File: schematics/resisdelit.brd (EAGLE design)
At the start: 10 x 14 mm, 7 parts

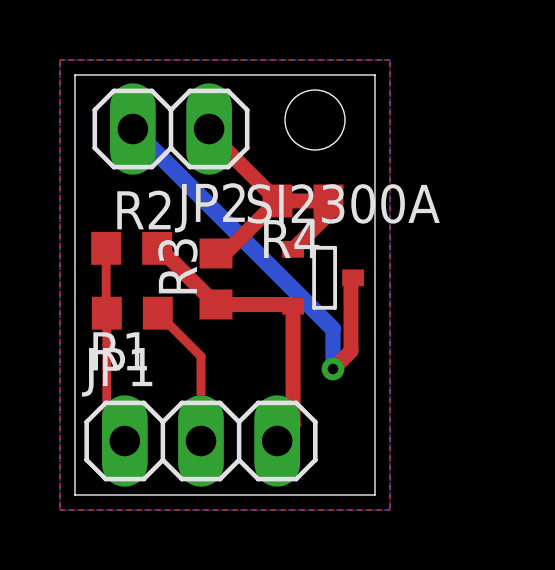
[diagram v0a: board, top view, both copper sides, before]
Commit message: заказ плат
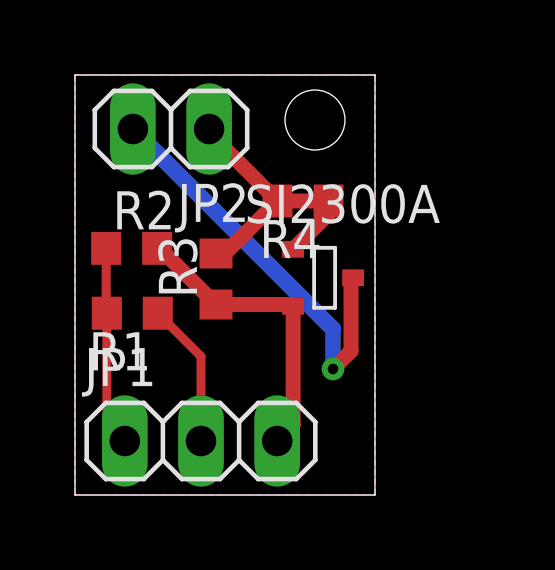
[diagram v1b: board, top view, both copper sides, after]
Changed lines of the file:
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@@
 <?xml version="1.0" encoding="utf-8"?>
 <!DOCTYPE eagle SYSTEM "eagle.dtd">
-<eagle version="9.6.2">
+<eagle version="9.4.2">
 <drawing>
 <settings>
-<setting alwaysvectorfont="no"/>
+<setting alwaysvectorfont="yes"/>
 <setting verticaltext="up"/>
 </settings>
@@
 <layer number="23" name="tOrigins" color="15" fill="1" visible="yes" active="yes"/>
 <layer number="24" name="bOrigins" color="15" fill="1" visible="yes" active="yes"/>
-<layer number="25" name="tNames" color="7" fill="1" visible="no" active="yes"/>
+<layer number="25" name="tNames" color="7" fill="1" visible="yes" active="yes"/>
 <layer number="26" name="bNames" color="7" fill="1" visible="yes" active="yes"/>
 <layer number="27" name="tValues" color="7" fill="1" visible="yes" active="yes"/>
 <layer number="28" name="bValues" color="7" fill="1" visible="yes" active="yes"/>
-<layer number="29" name="tStop" color="7" fill="3" visible="no" active="yes"/>
-<layer number="30" name="bStop" color="7" fill="6" visible="no" active="yes"/>
-<layer number="31" name="tCream" color="7" fill="4" visible="no" active="yes"/>
-<layer number="32" name="bCream" color="7" fill="5" visible="no" active="yes"/>
-<layer number="33" name="tFinish" color="6" fill="3" visible="no" active="yes"/>
-<layer number="34" name="bFinish" color="6" fill="6" visible="no" active="yes"/>
-<layer number="35" name="tGlue" color="7" fill="4" visible="no" active="yes"/>
-<layer number="36" name="bGlue" color="7" fill="5" visible="no" active="yes"/>
-<layer number="37" name="tTest" color="7" fill="1" visible="no" active="yes"/>
-<layer number="38" name="bTest" color="7" fill="1" visible="no" active="yes"/>
+<layer number="29" name="tStop" color="7" fill="3" visible="yes" active="yes"/>
+<layer number="30" name="bStop" color="7" fill="6" visible="yes" active="yes"/>
+<layer number="31" name="tCream" color="7" fill="4" visible="yes" active="yes"/>
+<layer number="32" name="bCream" color="7" fill="5" visible="yes" active="yes"/>
+<layer number="33" name="tFinish" color="6" fill="3" visible="yes" active="yes"/>
+<layer number="34" name="bFinish" color="6" fill="6" visible="yes" active="yes"/>
+<layer number="35" name="tGlue" color="7" fill="4" visible="yes" active="yes"/>
+<layer number="36" name="bGlue" color="7" fill="5" visible="yes" active="yes"/>
+<layer number="37" name="tTest" color="7" fill="1" visible="yes" active="yes"/>
+<layer number="38" name="bTest" color="7" fill="1" visible="yes" active="yes"/>
 <layer number="39" name="tKeepout" color="4" fill="11" visible="yes" active="yes"/>
 <layer number="40" name="bKeepout" color="1" fill="11" visible="yes" active="yes"/>
@@
 <layer number="42" name="bRestrict" color="1" fill="10" visible="yes" active="yes"/>
 <layer number="43" name="vRestrict" color="2" fill="10" visible="yes" active="yes"/>
-<layer number="44" name="Drills" color="7" fill="1" visible="no" active="yes"/>
+<layer number="44" name="Drills" color="7" fill="1" visible="yes" active="yes"/>
 <layer number="45" name="Holes" color="7" fill="1" visible="yes" active="yes"/>
-<layer number="46" name="Milling" color="3" fill="1" visible="no" active="yes"/>
-<layer number="47" name="Measures" color="7" fill="1" visible="no" active="yes"/>
+<layer number="46" name="Milling" color="3" fill="1" visible="yes" active="yes"/>
+<layer number="47" name="Measures" color="7" fill="1" visible="yes" active="yes"/>
 <layer number="48" name="Document" color="7" fill="1" visible="yes" active="yes"/>
 <layer number="49" name="Reference" color="7" fill="1" visible="yes" active="yes"/>
@@
 <layer number="111" name="111" color="7" fill="1" visible="no" active="no"/>
 <layer number="112" name="tSilk" color="7" fill="1" visible="no" active="no"/>
-<layer number="113" name="IDFDebug" color="7" fill="1" visible="no" active="yes"/>
+<layer number="113" name="IDFDebug" color="7" fill="1" visible="yes" active="yes"/>
 <layer number="114" name="Badge_Outline" color="7" fill="1" visible="no" active="no"/>
 <layer number="115" name="ReferenceISLANDS" color="7" fill="1" visible="no" active="no"/>
@@
 <layer number="223" name="223bmp" color="24" fill="1" visible="no" active="no"/>
 <layer number="224" name="224bmp" color="25" fill="1" visible="no" active="no"/>
-<layer number="225" name="225bmp" color="7" fill="1" visible="no" active="yes"/>
-<layer number="226" name="226bmp" color="7" fill="1" visible="no" active="yes"/>
-<layer number="227" name="227bmp" color="7" fill="1" visible="no" active="yes"/>
-<layer number="228" name="228bmp" color="7" fill="1" visible="no" active="yes"/>
+<layer number="225" name="225bmp" color="7" fill="1" visible="yes" active="yes"/>
+<layer number="226" name="226bmp" color="7" fill="1" visible="yes" active="yes"/>
+<layer number="227" name="227bmp" color="7" fill="1" visible="yes" active="yes"/>
+<layer number="228" name="228bmp" color="7" fill="1" visible="yes" active="yes"/>
 <layer number="229" name="229bmp" color="7" fill="1" visible="no" active="no"/>
-<layer number="230" name="230bmp" color="7" fill="1" visible="no" active="yes"/>
+<layer number="230" name="230bmp" color="7" fill="1" visible="yes" active="yes"/>
 <layer number="231" name="231bmp" color="7" fill="1" visible="no" active="no"/>
 <layer number="232" name="Eagle3D_PG2" color="7" fill="1" visible="no" active="no"/>
@@
 <wire x1="7.27" y1="2.33" x2="6.74" y2="1.8" width="0.5" layer="1"/>
 <polygon width="0.2" layer="1">
-<vertex x="-0.5" y="14.5"/>
-<vertex x="-0.5" y="-0.5"/>
-<vertex x="10.5" y="-0.5"/>
-<vertex x="10.5" y="14.5"/>
+<vertex x="0" y="14"/>
+<vertex x="0" y="0"/>
+<vertex x="10" y="0"/>
+<vertex x="10" y="14"/>
 </polygon>
 <polygon width="0.2" layer="16">
-<vertex x="-0.5" y="14.5"/>
-<vertex x="10.5" y="14.5"/>
-<vertex x="10.5" y="-0.5"/>
-<vertex x="-0.5" y="-0.5"/>
+<vertex x="0" y="14"/>
+<vertex x="10" y="14"/>
+<vertex x="10" y="0"/>
+<vertex x="0" y="0"/>
 </polygon>
 </signal>
